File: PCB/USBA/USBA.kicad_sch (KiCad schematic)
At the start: 19 parts, among them J1 USB_A, J2 Shelly, U1 ESP32-PICO-MINI-02, U2 LMR16006+FB, U4 QR

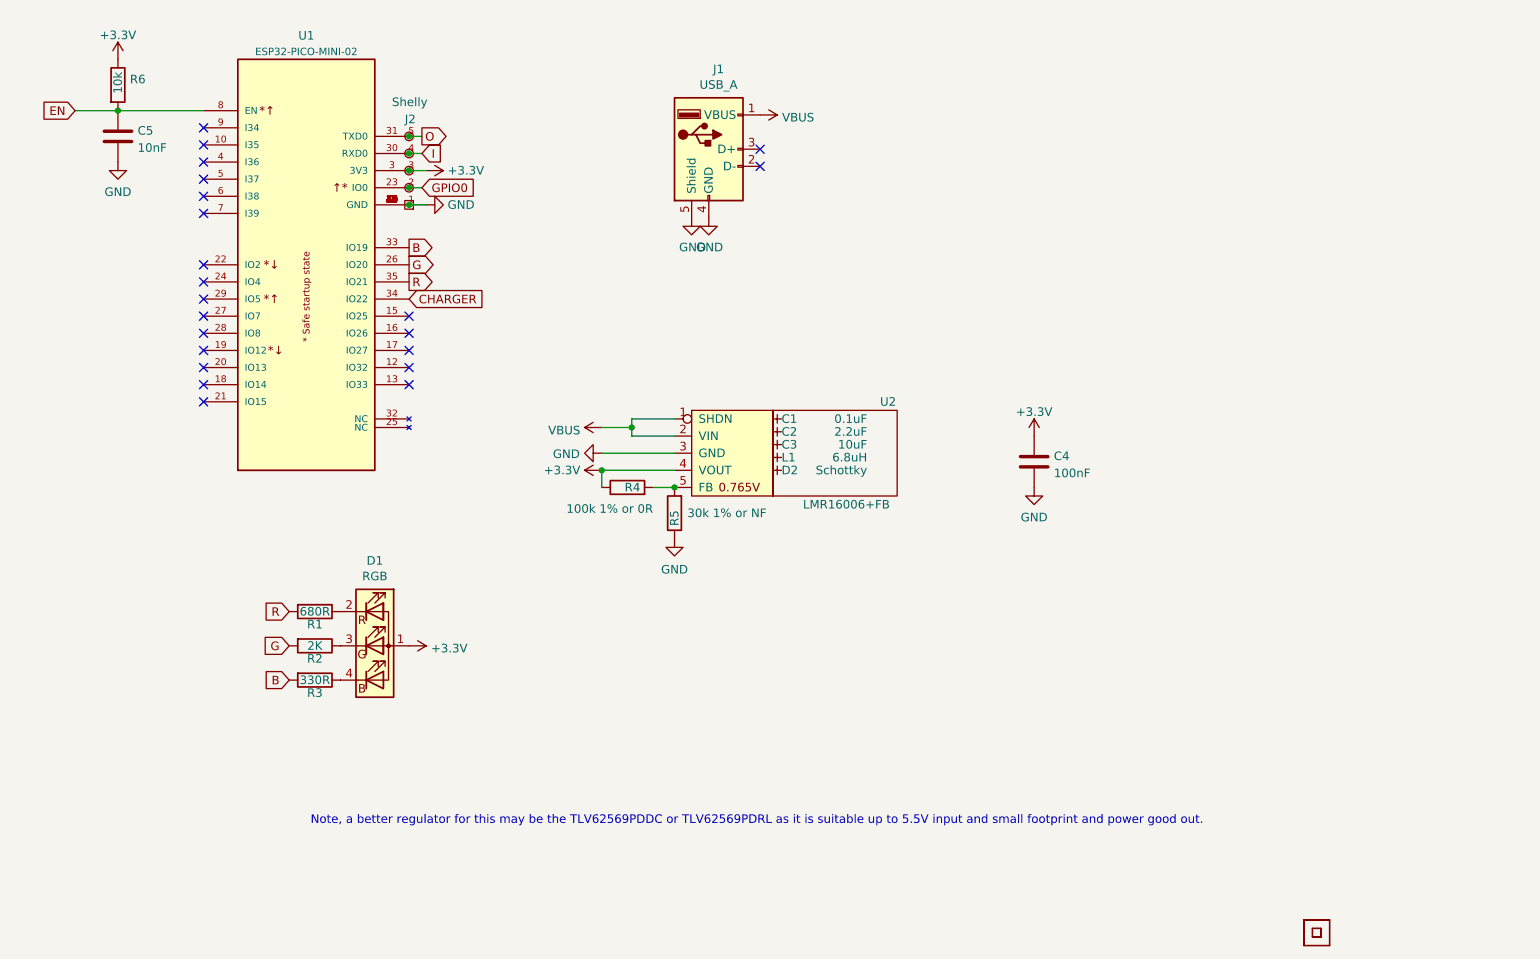
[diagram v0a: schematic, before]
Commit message: New layout for production
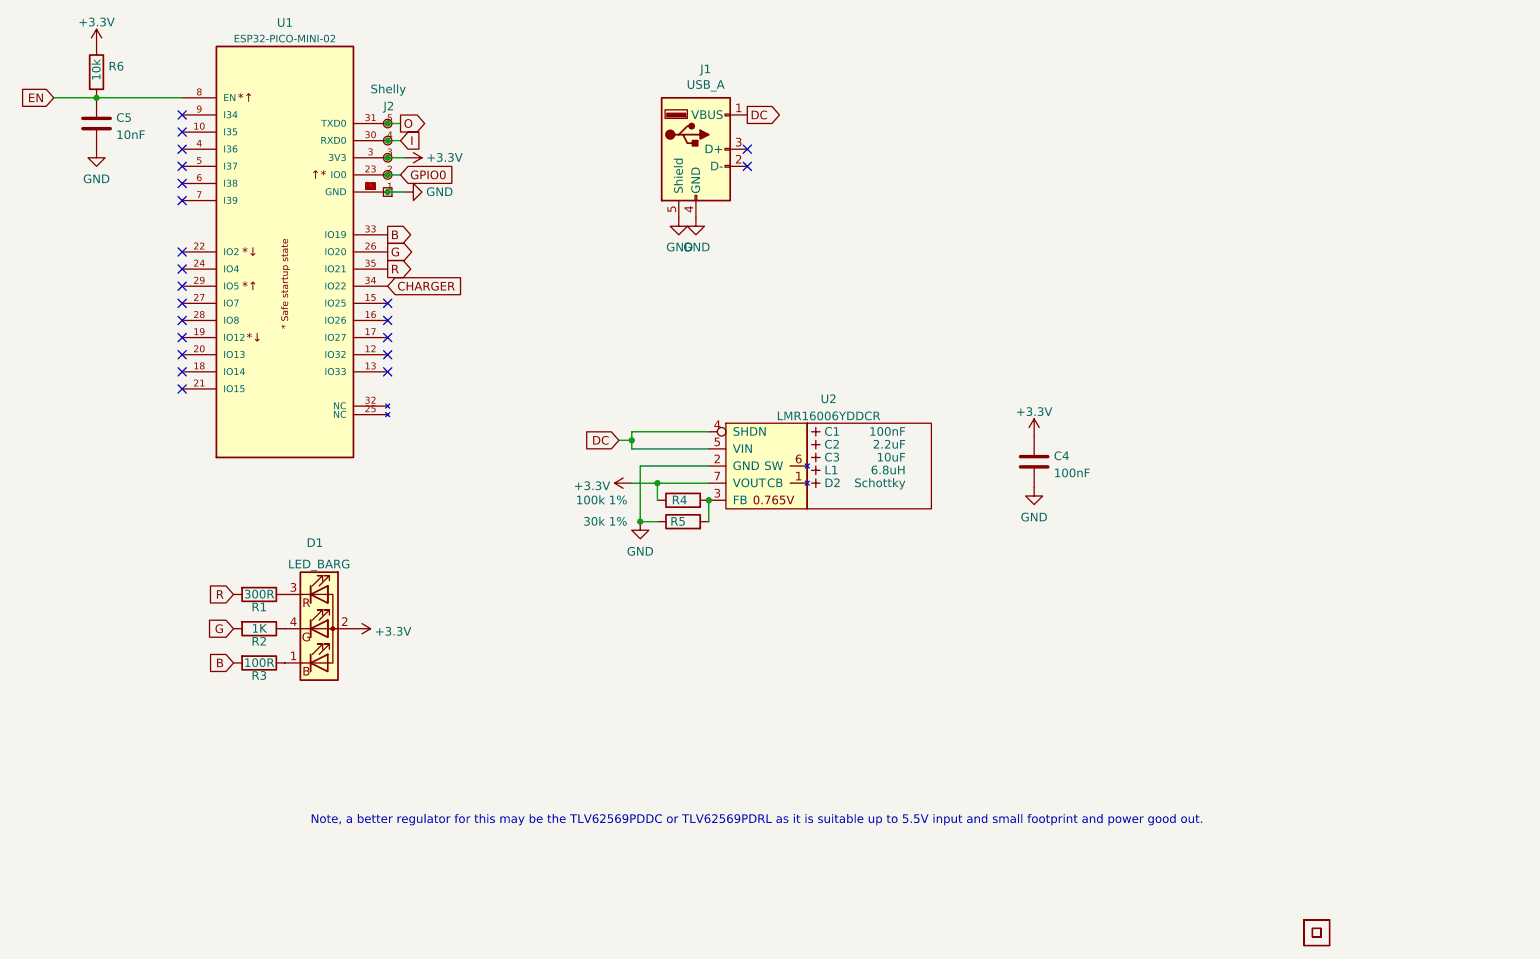
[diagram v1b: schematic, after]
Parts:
- removed D1: RGB, RevK:LED-RGB-1.6x1.6, symbol Device:LED_ARGB
- removed U2: LMR16006+FB, RevK:SOT-23-Thin-6-Reg, symbol RevK:LMR16006+FB
- added D1: LED_BARG, RevK:MHS190RGBCT, symbol Device:LED_BARG
- added U2: LMR16006YDDCR, RevK:SOT-23-Thin-6-Reg, symbol RevK:LMR16006XDDCR
- C1: value 0.1uF -> 100nF; LCSC Part # (none) -> C30926; Part No 0603-100nF-50V -> (none)
- C2: LCSC Part # (none) -> C19110; Note 0603 or 0805 -> (none); Part No 0805-2.2uF-25V -> (none)
- C3: LCSC Part # (none) -> C17024; Note 0603 or 0805 -> (none); Part No 0805-10uF-16V -> (none)
- D2: JLCPCB Rotation Offset (none) -> 0; LCSC Part # (none) -> C143805; Part No CD1206-B2100 -> (none)
- J1, U4: now left out of the parts list
- L1: LCSC Part # (none) -> C354575; Manufacturer Laird -> (none); Part No TYA40206R8M-10 -> (none)
- R1: value 680R -> 300R; Part No (none) -> 0603-680R
- R2: value 2K -> 1K; Part No (none) -> 0603-2K
- R3: value 330R -> 100R; Part No (none) -> 0603-220R
- R4: value 100k 1% or 0R -> 100k 1%; LCSC Part # (none) -> C14675; Part No 0603-100k -> (none)
- R5: value 30k 1% or NF -> 30k 1%; LCSC Part # (none) -> C100001; Part No 0603-30k -> (none)
- U1: JLCPCB Rotation Offset (none) -> 180; LCSC Part # (none) -> C2980306
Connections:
- net +3.3V: now also D1.2 (A), U2.7 (VOUT)
- net GND: now also U2.2 (GND)
- net at R3.1: now also D1.1 (BK)
- net at R1.1: now also D1.3 (RK)
- net at R2.1: now also D1.4 (GK)
- net at R4.2, R5.2: now also U2.3 (FB)
- net VBUS renamed DC
- net DC: now also U2.4 (SHDN), U2.5 (VIN)
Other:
- moved on the sheet: C5, J1, J2, R6, U1
